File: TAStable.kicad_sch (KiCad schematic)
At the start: 18 parts, among them J1 Conn_01x06_Pin, J2 ICSP, U1 74HCT1G04, U2 CS2300-CP, U3 74LVC1G14, U4 PIC16LF15313, U6 AZ1117-3.3

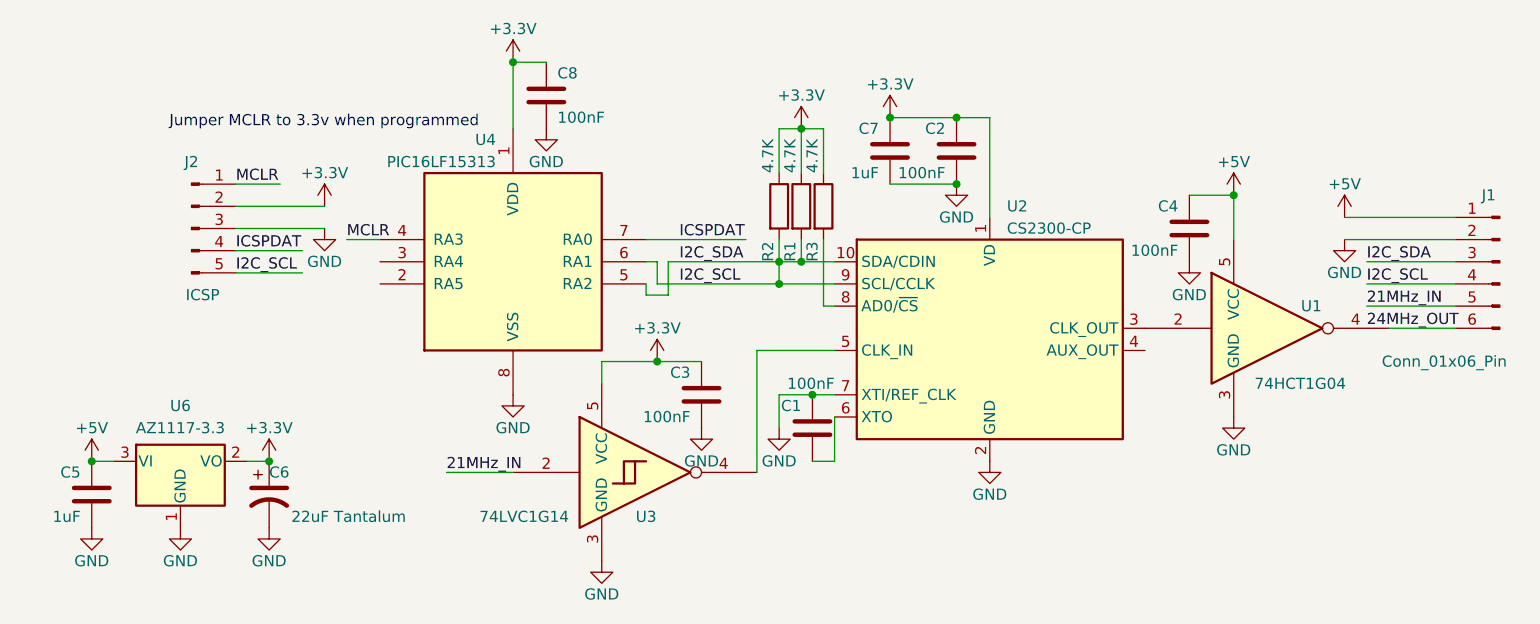
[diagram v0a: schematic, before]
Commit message: more pics + cleanups
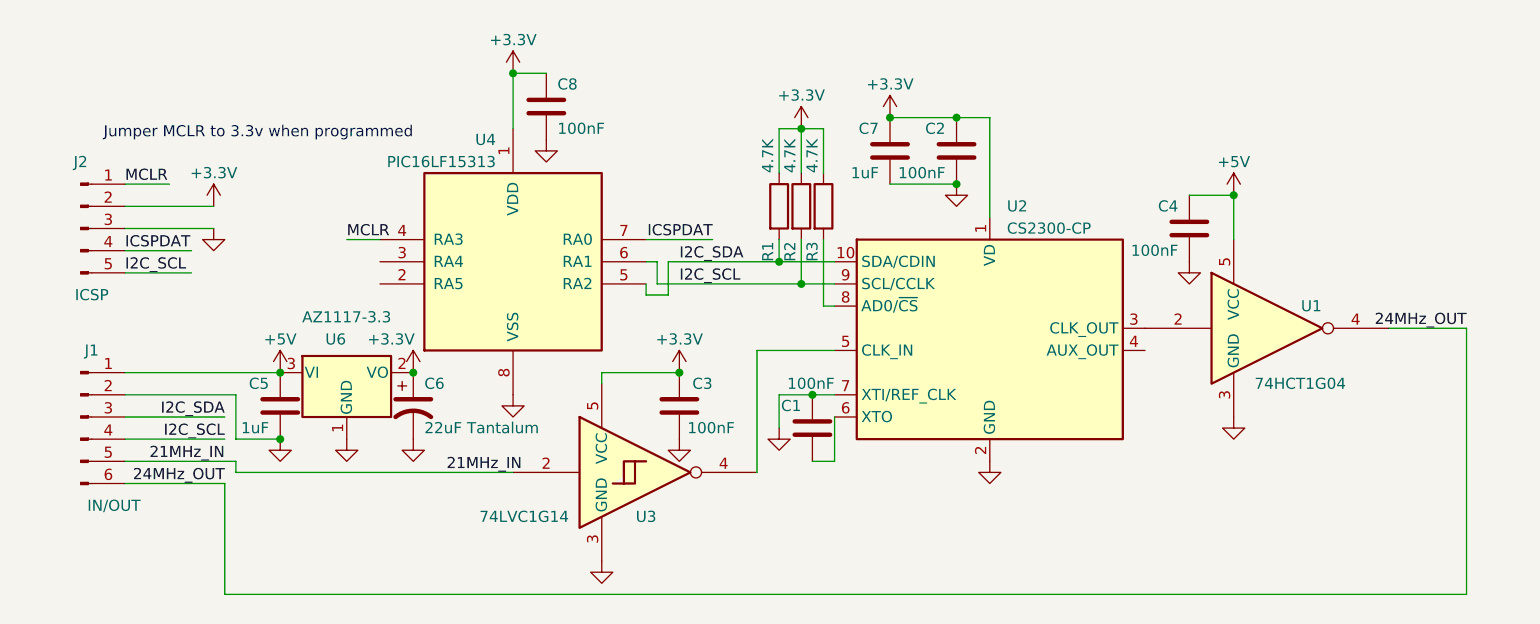
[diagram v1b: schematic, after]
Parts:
- J1: value Conn_01x06_Pin -> IN/OUT
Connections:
- net 24MHz_OUT: now also J1.6 (Pin_6), U1.4
- net I2C_SCL: no longer J1.3 (Pin_3), R1.2, U2.10 (SDA/CDIN), U4.5 (RA2)
- new net I2C_SDA: J1.3 (Pin_3), R1.2, U2.10 (SDA/CDIN), U4.5 (RA2)
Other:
- moved on the sheet: C3, C5, C6, C8, J1, J2, R1, R2, U6
